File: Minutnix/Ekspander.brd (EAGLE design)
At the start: 215.2 x 22 mm, 14 parts, among them X1 FH12-12S-0.5S_THINNER, X6 JST-XH-03-PIN-LONG-PAD

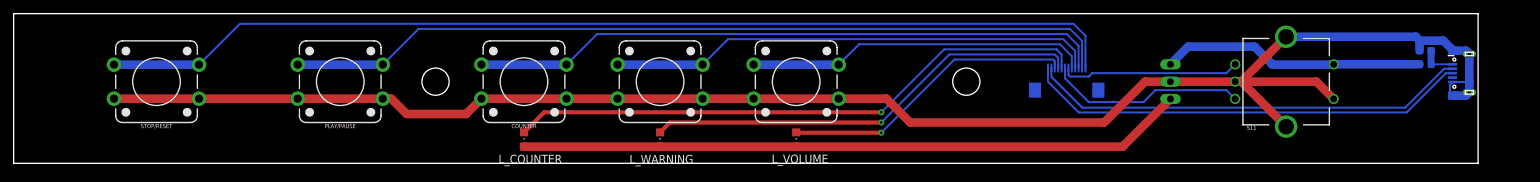
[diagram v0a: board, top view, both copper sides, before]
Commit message: lib update + board ongoing
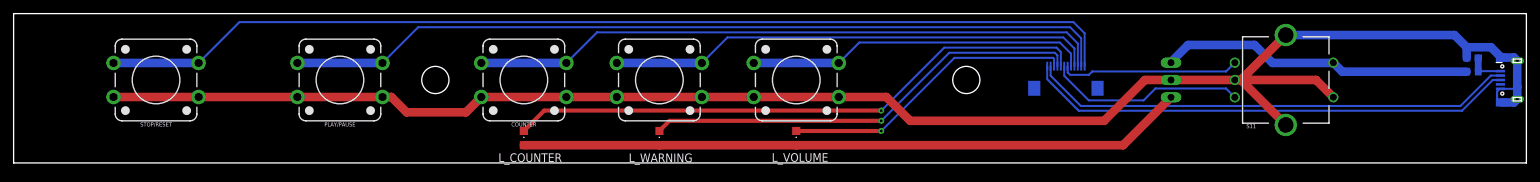
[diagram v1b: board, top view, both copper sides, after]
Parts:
- moved U$1 7.12 mm to (221.3, -9.75)
- moved L1 7.01 mm to (214.4, -8.53)
- moved C4 7.01 mm to (214.4, -6.50)
- moved X1 0.30 mm to (154.6, -11.0)
- moved WARNING 0.27 mm to (94.9, -9.75)
- moved X6 0.26 mm to (170.1, -9.75)
- moved STOP/RESET 0.26 mm to (20.9, -9.75)
- moved S11 0.25 mm to (186.9, -9.75)
- moved PLAY/PAUSE 0.25 mm to (48.0, -9.75)
- moved COUNTER 0.25 mm to (75.0, -9.75)
- moved VOLUME 0.25 mm to (115.0, -9.75)
- moved L_WARNING 0.24 mm to (94.9, -18.3)
- moved L_COUNTER 0.21 mm to (75.0, -18.3)
- moved L_VOLUME 0.21 mm to (115.0, -18.3)
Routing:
- net GND: track 248.1 -> 256.1 mm
- net +5V: track 38.8 -> 46.2 mm
- net N$7: track 64.5 -> 71.2 mm
- net N$9: track 65.7 -> 72.3 mm
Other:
- board size 215.2 x 22 mm -> 222.3 x 21.9 mm
